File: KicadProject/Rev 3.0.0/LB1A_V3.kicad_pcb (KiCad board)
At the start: 6 copper layers, 45 x 45 mm, 193 parts, among them J601 2337019-1, J602 2337019-1, U101 LFBGA448_18X18, U201 AS4C256M16D3LC-12BCN, U401 STPMIC1xPQR, U501 S40FC004C1B2C00000, U601 LBEE59B1LV-278, U701 DF40C-100DP-0.4V(51), U702 DF40C-100DP-0.4V(51), U703 DF40C-100DP-0.4V(51), X101 32.768kHz, Y101 24MHz

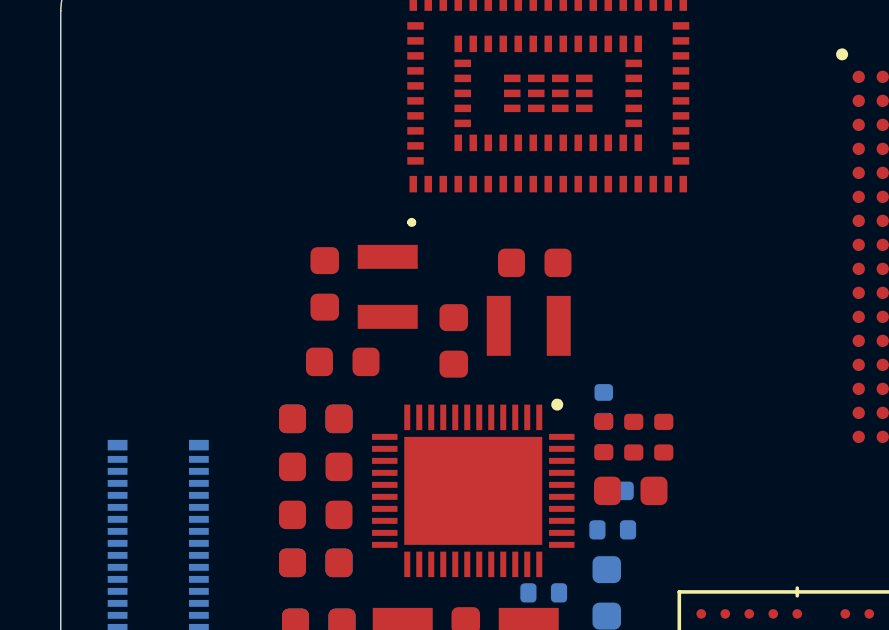
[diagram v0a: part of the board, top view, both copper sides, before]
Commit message: pmic complete
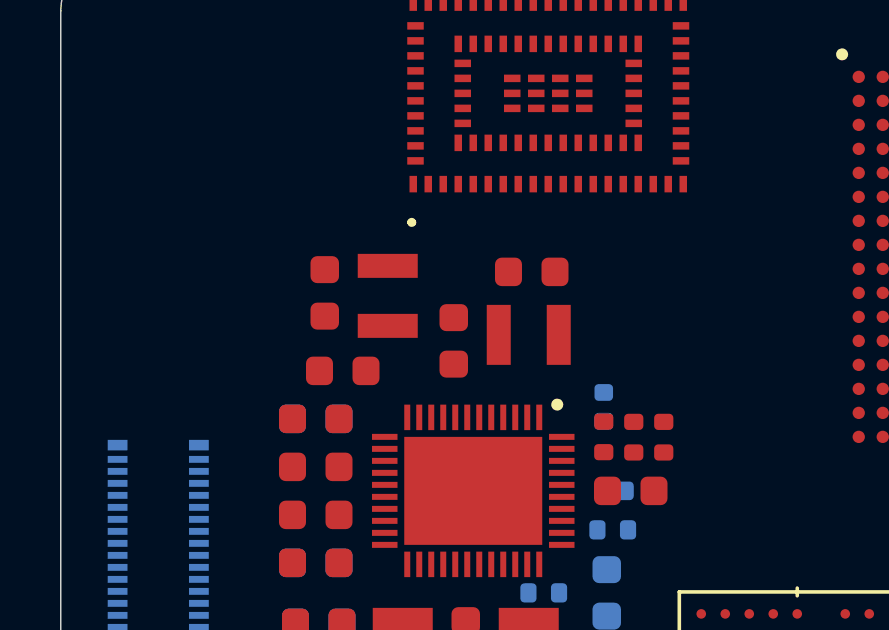
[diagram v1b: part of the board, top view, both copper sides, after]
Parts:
- moved C418 0.32 mm to (115.7, 95.7)
- moved C419 0.30 mm to (108.8, 96.4)
- moved C402 0.30 mm to (109.4, 99.0)
- moved L401 0.30 mm to (115.6, 97.8)
- moved L402 0.30 mm to (110.9, 96.5)
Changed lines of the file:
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@@
   )
   (module U_Inductor_SMD:MGV2520101R0M-10 (layer L1_Sig_Pwr.Cu)
-    (at 110.9 96.2 90)
+    (at 110.9 96.5 90)
     (fp_text reference L402 (at 0.382 -1.9064 90) (layer F.SilkS) hide
       (effects (font (size 0.6 0.6) (thickness 0.09)))
@@
   )
   (module U_Inductor_SMD:MGV2520101R0M-10 (layer L1_Sig_Pwr.Cu)
-    (at 115.6 97.5)
+    (at 115.6 97.8)
     (fp_text reference L401 (at 0.382 -1.9064) (layer F.SilkS) hide
       (effects (font (size 0.6 0.6) (thickness 0.09)))
@@
   )
   (module U_Capacitor_SMD:C_0603_1608Metric (layer L1_Sig_Pwr.Cu)
-    (at 108.8 96.1 270)
+    (at 108.8 96.4 270)
     (descr "Capacitor SMD 0603 (1608 Metric), square (rectangular) end terminal, IPC_7351 nominal, (Body size source: IPC-SM-782 page 76, https://www.pcb-3d.com/wordpress/wp-content/uploads/ipc-sm-782a_amendment_1_and_2.pdf), generated with kicad-footprint-generator")
     (tags capacitor)
@@
   )
   (module U_Capacitor_SMD:C_0603_1608Metric (layer L1_Sig_Pwr.Cu)
-    (at 115.8 95.4 180)
+    (at 115.7 95.7 180)
     (descr "Capacitor SMD 0603 (1608 Metric), square (rectangular) end terminal, IPC_7351 nominal, (Body size source: IPC-SM-782 page 76, https://www.pcb-3d.com/wordpress/wp-content/uploads/ipc-sm-782a_amendment_1_and_2.pdf), generated with kicad-footprint-generator")
     (tags capacitor)
@@
   )
   (module U_Capacitor_SMD:C_0603_1608Metric (layer L1_Sig_Pwr.Cu)
-    (at 109.4 98.7 180)
-    (descr "Capacitor SMD 0603 (1608 Metric), square (rectangular) end terminal, IPC_7351 nominal, (Body size source: IPC-SM-782 page 76, https://www.pcb-3d.com/wordpress/wp-content/uploads/ipc-sm-782a_amendment_1_and_2.pdf), generated with kicad-footprint-generator")
-    (tags capacitor)
+    (at 109.4 99 180)
+    (descr "Capacitor SMD 0603 (1608 Metric), square (rectangular) end terminal, IPC_7351 nominal, (Body size source: IPC-SM-782 page 76, https://www.pcb-3d.com/wordpress/wp-content/uploads/ipc-sm-782a_amendment_1_and_2.pdf), generated with kicad-footprint-generator")
+    (tags capacitor)
